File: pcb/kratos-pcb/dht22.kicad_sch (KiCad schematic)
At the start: 3 parts, among them U2 DHT22

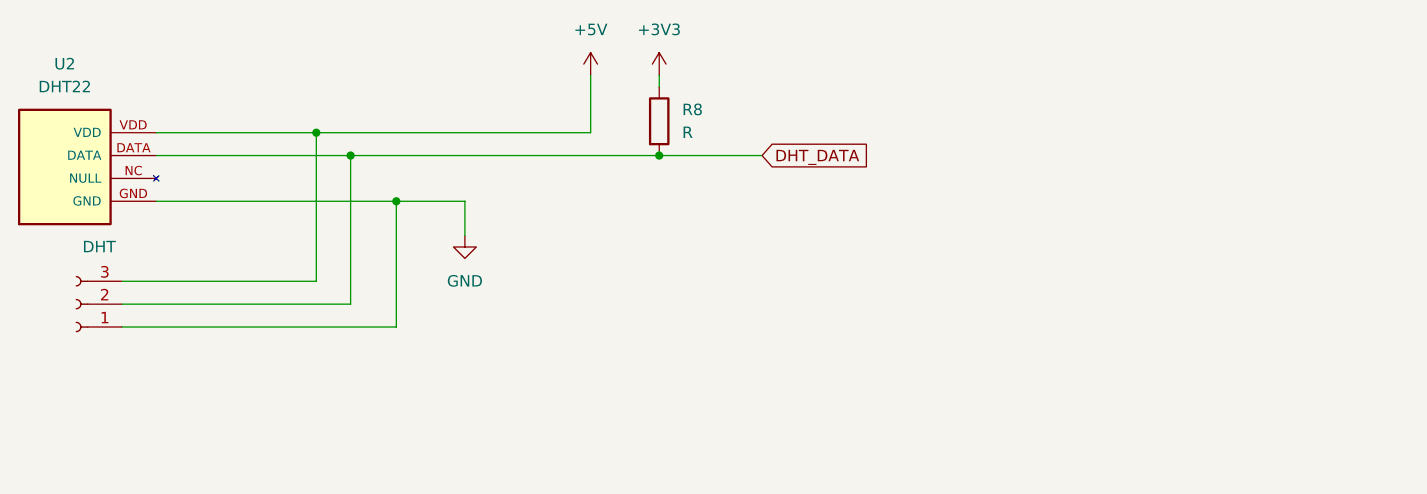
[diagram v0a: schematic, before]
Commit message: ### added
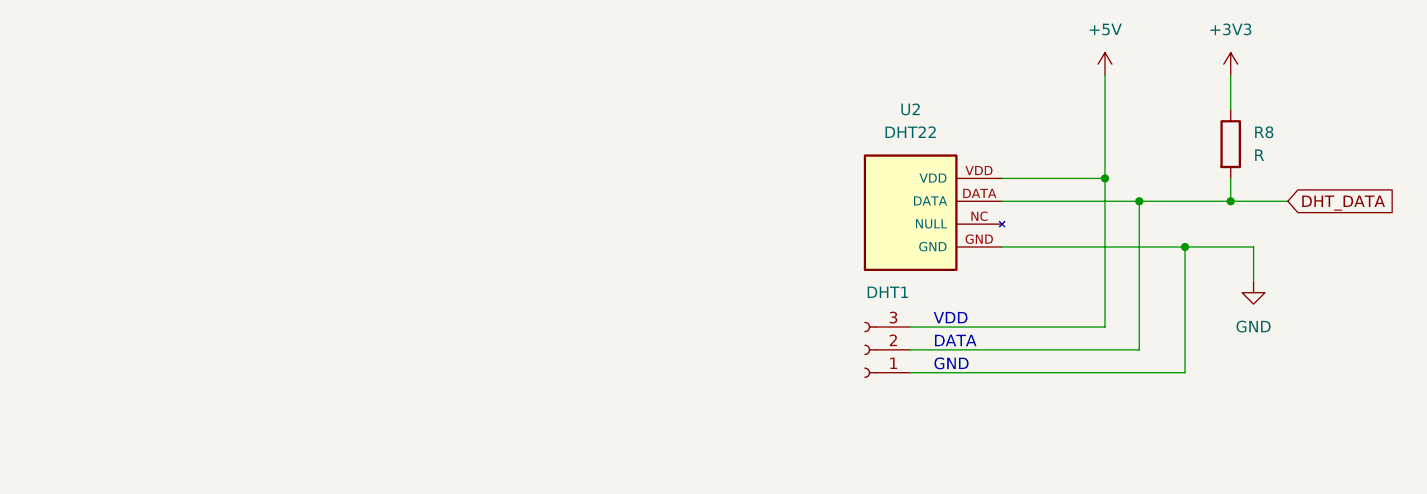
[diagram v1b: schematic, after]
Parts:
- DHT1: renamed from DHT; footprint (none) -> Connector:JWT_A3963_1x02_P3.96mm_Vertical
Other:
- note added: "DATA"
- note added: "GND"
- note added: "VDD"
- moved on the sheet: DHT1, R8, U2

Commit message: ### update     - kicad schematic
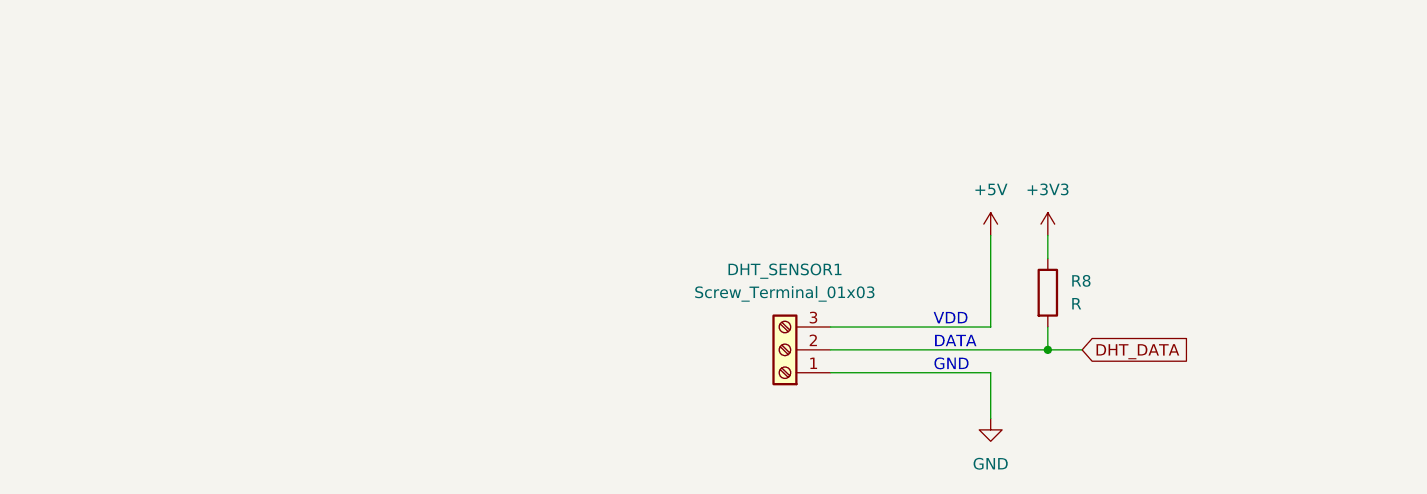
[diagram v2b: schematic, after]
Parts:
- removed DHT1: Conn_01x03_Socket, Connector:JWT_A3963_1x02_P3.96mm_Vertical, symbol Connector:Conn_01x03_Socket
- removed U2: DHT22, DHT22:DHT22, symbol DHT22:DHT22
- added DHT_SENSOR1: Screw_Terminal_01x03, TerminalBlock_4Ucon:TerminalBlock_4Ucon_1x03_P3.50mm_Horizontal, symbol Connector:Screw_Terminal_01x03
- R8: footprint (none) -> Resistor_THT:R_Axial_DIN0204_L3.6mm_D1.6mm_P5.08mm_Horizontal
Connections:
- net +5V: now also DHT_SENSOR1.3 (Pin_3)
- net DHT_DATA: now also DHT_SENSOR1.2 (Pin_2)
- net GND: now also DHT_SENSOR1.1 (Pin_1)
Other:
- moved on the sheet: R8
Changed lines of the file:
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@@
 (kicad_sch (version 20230121) (generator eeschema)
   (paper "A4")
-  (junction (at 151.13 95.25) (diameter 0) (color 0 0 0 0)
+  (junction (at 135.89 106.68) (diameter 0) (color 0 0 0 0)
   )
-  (junction (at 156.21 90.17) (diameter 0) (color 0 0 0 0)
-  )
-  (junction (at 142.24 87.63) (diameter 0) (color 0 0 0 0)
-  )
-  (junction (at 146.05 90.17) (diameter 0) (color 0 0 0 0)
-  )
-  (wire (pts (xy 146.05 106.68) (xy 146.05 90.17))
+  (wire (pts (xy 135.89 106.68) (xy 139.7 106.68))
     (stroke (width 0) (type default))
   )
-  (wire (pts (xy 120.65 104.14) (xy 142.24 104.14))
+  (wire (pts (xy 135.89 93.98) (xy 135.89 96.52))
     (stroke (width 0) (type default))
   )
-  (wire (pts (xy 130.81 90.17) (xy 146.05 90.17))
+  (wire (pts (xy 111.76 106.68) (xy 135.89 106.68))
     (stroke (width 0) (type default))
   )
-  (wire (pts (xy 151.13 95.25) (xy 130.81 95.25))
+  (wire (pts (xy 111.76 104.14) (xy 129.54 104.14))
     (stroke (width 0) (type default))
   )
-  (wire (pts (xy 130.81 87.63) (xy 142.24 87.63))
+  (wire (pts (xy 111.76 109.22) (xy 129.54 109.22))
     (stroke (width 0) (type default))
   )
-  (wire (pts (xy 146.05 90.17) (xy 156.21 90.17))
+  (wire (pts (xy 129.54 93.98) (xy 129.54 104.14))
     (stroke (width 0) (type default))
   )
-  (wire (pts (xy 120.65 109.22) (xy 151.13 109.22))
+  (wire (pts (xy 135.89 104.14) (xy 135.89 106.68))
     (stroke (width 0) (type default))
   )
-  (wire (pts (xy 142.24 87.63) (xy 142.24 76.2))
-    (stroke (width 0) (type default))
-  )
-  (wire (pts (xy 120.65 106.68) (xy 146.05 106.68))
-    (stroke (width 0) (type default))
-  )
-  (wire (pts (xy 142.24 104.14) (xy 142.24 87.63))
-    (stroke (width 0) (type default))
-  )
-  (wire (pts (xy 151.13 109.22) (xy 151.13 95.25))
-    (stroke (width 0) (type default))
-  )
-  (wire (pts (xy 158.75 95.25) (xy 151.13 95.25))
-    (stroke (width 0) (type default))
-  )
-  (wire (pts (xy 156.21 87.63) (xy 156.21 90.17))
-    (stroke (width 0) (type default))
-  )
-  (wire (pts (xy 156.21 90.17) (xy 162.56 90.17))
-    (stroke (width 0) (type default))
-  )
-  (wire (pts (xy 158.75 95.25) (xy 158.75 99.06))
-    (stroke (width 0) (type default))
-  )
-  (wire (pts (xy 156.21 76.2) (xy 156.21 80.01))
+  (wire (pts (xy 129.54 109.22) (xy 129.54 114.3))
     (stroke (width 0) (type default))
   )
@@
     (effects (font (size 1.27 1.27)) (justify left bottom))
   )
-  (global_label "DHT_DATA" (shape input) (at 162.56 90.17 0) (fields_autoplaced)
+  (global_label "DHT_DATA" (shape input) (at 139.7 106.68 0) (fields_autoplaced)
     (effects (font (size 1.27 1.27)) (justify left))
-    (property "Intersheetrefs" "${INTERSHEET_REFS}" (at 174.4957 90.17 0)
+    (property "Intersheetrefs" "${INTERSHEET_REFS}" (at 151.6357 106.68 0)
       (effects (font (size 1.27 1.27)) (justify left) hide)
     )
   )
-  (symbol (lib_id "power:GND") (at 158.75 99.06 0) (unit 1)
+  (symbol (lib_id "power:GND") (at 129.54 114.3 0) (unit 1)
     (in_bom yes) (on_board yes) (dnp no) (fields_autoplaced)
-    (property "Reference" "#PWR014" (at 158.75 105.41 0)
+    (property "Reference" "#PWR014" (at 129.54 120.65 0)
       (effects (font (size 1.27 1.27)) hide)
     )
-    (property "Value" "GND" (at 158.75 104.14 0)
+    (property "Value" "GND" (at 129.54 119.38 0)
       (effects (font (size 1.27 1.27)))
     )
-    (property "Footprint" "" (at 158.75 99.06 0)
+    (property "Footprint" "" (at 129.54 114.3 0)
       (effects (font (size 1.27 1.27)) hide)
     )
-    (property "Datasheet" "" (at 158.75 99.06 0)
+    (property "Datasheet" "" (at 129.54 114.3 0)
       (effects (font (size 1.27 1.27)) hide)
     )
@@
     )
   )
-  (symbol (lib_id "DHT22:DHT22") (at 115.57 97.79 0) (unit 1)
+  (symbol (lib_id "Connector:Screw_Terminal_01x03") (at 106.68 106.68 180) (unit 1)
     (in_bom yes) (on_board yes) (dnp no) (fields_autoplaced)
-    (property "Reference" "U2" (at 120.65 80.01 0)
+    (property "Reference" "DHT_SENSOR1" (at 106.68 97.79 0)
       (effects (font (size 1.27 1.27)))
     )
-    (property "Value" "DHT22" (at 120.65 82.55 0)
+    (property "Value" "Screw_Terminal_01x03" (at 106.68 100.33 0)
       (effects (font (size 1.27 1.27)))
     )
-    (property "Footprint" "DHT22:DHT22" (at 115.57 97.79 0)
-      (effects (font (size 1.27 1.27)) (justify bottom) hide)
-    )
-    (property "Datasheet" "" (at 115.57 97.79 0)
+    (property "Footprint" "TerminalBlock_4Ucon:TerminalBlock_4Ucon_1x03_P3.50mm_Horizontal" (at 106.68 106.68 0)
       (effects (font (size 1.27 1.27)) hide)
     )
-    (property "MF" "Aosong Electronics" (at 115.57 97.79 0)
-      (effects (font (size 1.27 1.27)) (justify bottom) hide)
+    (property "Datasheet" "~" (at 106.68 106.68 0)
+      (effects (font (size 1.27 1.27)) hide)
     )
-    (property "Description" "\nCapacitive-type humidity and temperature module/sensor\n" (at 115.57 97.79 0)
-      (effects (font (size 1.27 1.27)) (justify bottom) hide)
-    )
-    (property "Package" "Package" (at 115.57 97.79 0)
-      (effects (font (size 1.27 1.27)) (justify bottom) hide)
-    )
-    (property "Price" "None" (at 115.57 97.79 0)
-      (effects (font (size 1.27 1.27)) (justify bottom) hide)
-    )
-    (property "SnapEDA_Link" "https://www.snapeda.com/parts/DHT22/Aosong+Electronics/view-part/?ref=snap" (at 115.57 97.79 0)
-      (effects (font (size 1.27 1.27)) (justify bottom) hide)
-    )
-    (property "MP" "DHT22" (at 115.57 97.79 0)
-      (effects (font (size 1.27 1.27)) (justify bottom) hide)
-    )
-    (property "Availability" "Not in stock" (at 115.57 97.79 0)
-      (effects (font (size 1.27 1.27)) (justify bottom) hide)
-    )
-    (property "Check_prices" "https://www.snapeda.com/parts/DHT22/Aosong+Electronics/view-part/?ref=eda" (at 115.57 97.79 0)
-      (effects (font (size 1.27 1.27)) (justify bottom) hide)
-    )
-    (pin "DATA")
-    (pin "GND")
-    (pin "NC")
-    (pin "VDD")
+    (pin "2")
+    (pin "1")
+    (pin "3")
     (instances
       (project "kratos-pcb"
         (path "/12f1b997-8c5f-4ef7-b036-7873ddaba48e/ab0aa194-5f27-4f16-bd8b-12afa764e651"
-          (reference "U2") (unit 1)
+          (reference "DHT_SENSOR1") (unit 1)
         )
       )
     )
   )
-  (symbol (lib_id "Connector:Conn_01x03_Socket") (at 115.57 106.68 180) (unit 1)
-    (in_bom yes) (on_board yes) (dnp no)
-    (property "Reference" "DHT1" (at 118.11 100.33 0)
+  (symbol (lib_id "power:+3V3") (at 135.89 93.98 0) (unit 1)
+    (in_bom yes) (on_board yes) (dnp no) (fields_autoplaced)
+    (property "Reference" "#PWR012" (at 135.89 97.79 0)
+      (effects (font (size 1.27 1.27)) hide)
+    )
+    (property "Value" "+3V3" (at 135.89 88.9 0)
       (effects (font (size 1.27 1.27)))
     )
-    (property "Value" "Conn_01x03_Socket" (at 110.49 101.6 0)
+    (property "Footprint" "" (at 135.89 93.98 0)
       (effects (font (size 1.27 1.27)) hide)
     )
-    (property "Footprint" "Connector:JWT_A3963_1x02_P3.96mm_Vertical" (at 115.57 106.68 0)
-      (effects (font (size 1.27 1.27)) hide)
-    )
-    (property "Datasheet" "~" (at 115.57 106.68 0)
-      (effects (font (size 1.27 1.27)) hide)
-    )
-    (pin "3")
-    (pin "2")
-    (pin "1")
-    (instances
-      (project "kratos-pcb"
-        (path "/12f1b997-8c5f-4ef7-b036-7873ddaba48e/ab0aa194-5f27-4f16-bd8b-12afa764e651"
-          (reference "DHT1") (unit 1)
-        )
-      )
-    )
-  )
-  (symbol (lib_id "power:+3V3") (at 156.21 76.2 0) (unit 1)
-    (in_bom yes) (on_board yes) (dnp no) (fields_autoplaced)
-    (property "Reference" "#PWR012" (at 156.21 80.01 0)
-      (effects (font (size 1.27 1.27)) hide)
-    )
-    (property "Value" "+3V3" (at 156.21 71.12 0)
-      (effects (font (size 1.27 1.27)))
-    )
-    (property "Footprint" "" (at 156.21 76.2 0)
-      (effects (font (size 1.27 1.27)) hide)
-    )
-    (property "Datasheet" "" (at 156.21 76.2 0)
+    (property "Datasheet" "" (at 135.89 93.98 0)
       (effects (font (size 1.27 1.27)) hide)
     )
@@
     )
   )
-  (symbol (lib_id "Device:R") (at 156.21 83.82 0) (unit 1)
+  (symbol (lib_id "Device:R") (at 135.89 100.33 0) (unit 1)
     (in_bom yes) (on_board yes) (dnp no) (fields_autoplaced)
-    (property "Reference" "R8" (at 158.75 82.55 0)
+    (property "Reference" "R8" (at 138.43 99.06 0)
       (effects (font (size 1.27 1.27)) (justify left))
     )
-    (property "Value" "R" (at 158.75 85.09 0)
+    (property "Value" "R" (at 138.43 101.6 0)
       (effects (font (size 1.27 1.27)) (justify left))
     )
-    (property "Footprint" "" (at 154.432 83.82 90)
+    (property "Footprint" "Resistor_THT:R_Axial_DIN0204_L3.6mm_D1.6mm_P5.08mm_Horizontal" (at 134.112 100.33 90)
       (effects (font (size 1.27 1.27)) hide)
     )
-    (property "Datasheet" "~" (at 156.21 83.82 0)
+    (property "Datasheet" "~" (at 135.89 100.33 0)
       (effects (font (size 1.27 1.27)) hide)
     )
@@
     )
   )
-  (symbol (lib_id "power:+5V") (at 142.24 76.2 0) (unit 1)
+  (symbol (lib_id "power:+5V") (at 129.54 93.98 0) (unit 1)
     (in_bom yes) (on_board yes) (dnp no) (fields_autoplaced)
-    (property "Reference" "#PWR013" (at 142.24 80.01 0)
+    (property "Reference" "#PWR013" (at 129.54 97.79 0)
       (effects (font (size 1.27 1.27)) hide)
     )
-    (property "Value" "+5V" (at 142.24 71.12 0)
+    (property "Value" "+5V" (at 129.54 88.9 0)
       (effects (font (size 1.27 1.27)))
     )
-    (property "Footprint" "" (at 142.24 76.2 0)
+    (property "Footprint" "" (at 129.54 93.98 0)
       (effects (font (size 1.27 1.27)) hide)
     )
-    (property "Datasheet" "" (at 142.24 76.2 0)
+    (property "Datasheet" "" (at 129.54 93.98 0)
       (effects (font (size 1.27 1.27)) hide)
     )

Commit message: kicad
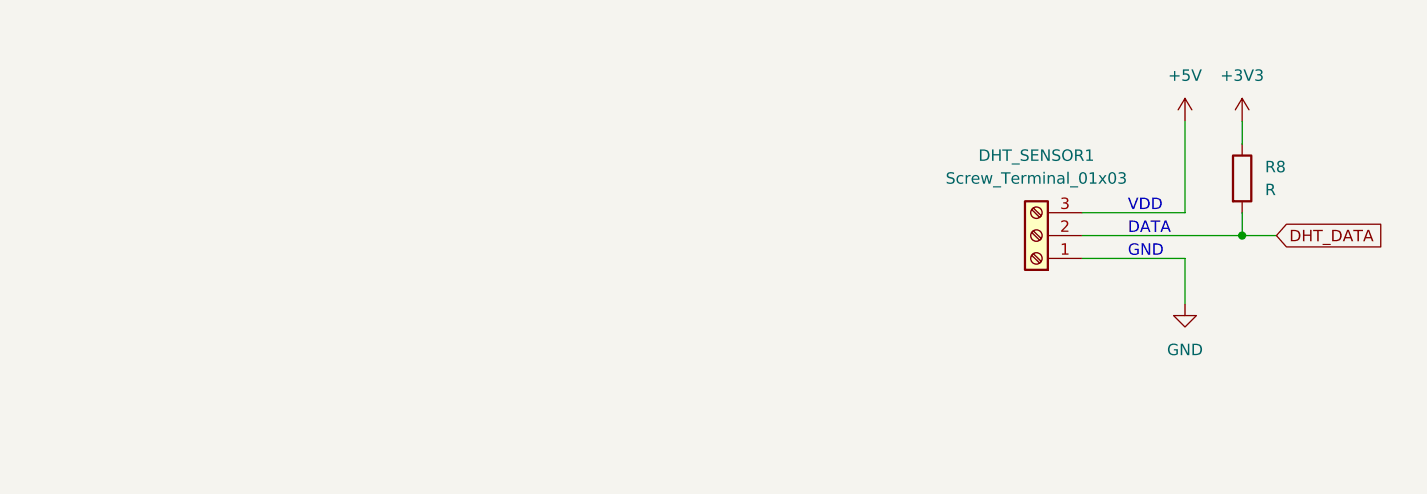
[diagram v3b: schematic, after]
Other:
- moved on the sheet: DHT_SENSOR1, R8
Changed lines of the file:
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@@
 (kicad_sch (version 20230121) (generator eeschema)
   (paper "A4")
-  (junction (at 135.89 106.68) (diameter 0) (color 0 0 0 0)
+  (junction (at 157.48 93.98) (diameter 0) (color 0 0 0 0)
   )
-  (wire (pts (xy 135.89 106.68) (xy 139.7 106.68))
+  (wire (pts (xy 157.48 81.28) (xy 157.48 83.82))
     (stroke (width 0) (type default))
   )
-  (wire (pts (xy 135.89 93.98) (xy 135.89 96.52))
+  (wire (pts (xy 139.7 93.98) (xy 157.48 93.98))
     (stroke (width 0) (type default))
   )
-  (wire (pts (xy 111.76 106.68) (xy 135.89 106.68))
+  (wire (pts (xy 139.7 91.44) (xy 151.13 91.44))
     (stroke (width 0) (type default))
   )
-  (wire (pts (xy 111.76 104.14) (xy 129.54 104.14))
+  (wire (pts (xy 157.48 93.98) (xy 161.29 93.98))
     (stroke (width 0) (type default))
   )
-  (wire (pts (xy 111.76 109.22) (xy 129.54 109.22))
+  (wire (pts (xy 139.7 96.52) (xy 151.13 96.52))
     (stroke (width 0) (type default))
   )
-  (wire (pts (xy 129.54 93.98) (xy 129.54 104.14))
+  (wire (pts (xy 151.13 81.28) (xy 151.13 91.44))
     (stroke (width 0) (type default))
   )
-  (wire (pts (xy 135.89 104.14) (xy 135.89 106.68))
+  (wire (pts (xy 157.48 91.44) (xy 157.48 93.98))
     (stroke (width 0) (type default))
   )
-  (wire (pts (xy 129.54 109.22) (xy 129.54 114.3))
+  (wire (pts (xy 151.13 96.52) (xy 151.13 101.6))
     (stroke (width 0) (type default))
   )
-  (text "VDD" (at 123.19 104.14 0)
+  (text "VDD" (at 144.78 91.44 0)
     (effects (font (size 1.27 1.27)) (justify left bottom))
   )
-  (text "DATA" (at 123.19 106.68 0)
+  (text "DATA" (at 144.78 93.98 0)
     (effects (font (size 1.27 1.27)) (justify left bottom))
   )
-  (text "GND" (at 123.19 109.22 0)
+  (text "GND" (at 144.78 96.52 0)
     (effects (font (size 1.27 1.27)) (justify left bottom))
   )
-  (global_label "DHT_DATA" (shape input) (at 139.7 106.68 0) (fields_autoplaced)
+  (global_label "DHT_DATA" (shape input) (at 161.29 93.98 0) (fields_autoplaced)
     (effects (font (size 1.27 1.27)) (justify left))
-    (property "Intersheetrefs" "${INTERSHEET_REFS}" (at 151.6357 106.68 0)
+    (property "Intersheetrefs" "${INTERSHEET_REFS}" (at 173.2257 93.98 0)
       (effects (font (size 1.27 1.27)) (justify left) hide)
     )
   )
-  (symbol (lib_id "power:GND") (at 129.54 114.3 0) (unit 1)
+  (symbol (lib_id "power:GND") (at 151.13 101.6 0) (unit 1)
     (in_bom yes) (on_board yes) (dnp no) (fields_autoplaced)
-    (property "Reference" "#PWR014" (at 129.54 120.65 0)
+    (property "Reference" "#PWR014" (at 151.13 107.95 0)
       (effects (font (size 1.27 1.27)) hide)
     )
-    (property "Value" "GND" (at 129.54 119.38 0)
+    (property "Value" "GND" (at 151.13 106.68 0)
       (effects (font (size 1.27 1.27)))
     )
-    (property "Footprint" "" (at 129.54 114.3 0)
+    (property "Footprint" "" (at 151.13 101.6 0)
       (effects (font (size 1.27 1.27)) hide)
     )
-    (property "Datasheet" "" (at 129.54 114.3 0)
+    (property "Datasheet" "" (at 151.13 101.6 0)
       (effects (font (size 1.27 1.27)) hide)
     )
@@
     )
   )
-  (symbol (lib_id "Connector:Screw_Terminal_01x03") (at 106.68 106.68 180) (unit 1)
+  (symbol (lib_id "Connector:Screw_Terminal_01x03") (at 134.62 93.98 180) (unit 1)
     (in_bom yes) (on_board yes) (dnp no) (fields_autoplaced)
-    (property "Reference" "DHT_SENSOR1" (at 106.68 97.79 0)
+    (property "Reference" "DHT_SENSOR1" (at 134.62 85.09 0)
       (effects (font (size 1.27 1.27)))
     )
-    (property "Value" "Screw_Terminal_01x03" (at 106.68 100.33 0)
+    (property "Value" "Screw_Terminal_01x03" (at 134.62 87.63 0)
       (effects (font (size 1.27 1.27)))
     )
-    (property "Footprint" "TerminalBlock_4Ucon:TerminalBlock_4Ucon_1x03_P3.50mm_Horizontal" (at 106.68 106.68 0)
+    (property "Footprint" "TerminalBlock_4Ucon:TerminalBlock_4Ucon_1x03_P3.50mm_Horizontal" (at 134.62 93.98 0)
       (effects (font (size 1.27 1.27)) hide)
     )
-    (property "Datasheet" "~" (at 106.68 106.68 0)
+    (property "Datasheet" "~" (at 134.62 93.98 0)
       (effects (font (size 1.27 1.27)) hide)
     )
@@
     )
   )
-  (symbol (lib_id "power:+3V3") (at 135.89 93.98 0) (unit 1)
+  (symbol (lib_id "power:+3V3") (at 157.48 81.28 0) (unit 1)
     (in_bom yes) (on_board yes) (dnp no) (fields_autoplaced)
-    (property "Reference" "#PWR012" (at 135.89 97.79 0)
+    (property "Reference" "#PWR012" (at 157.48 85.09 0)
       (effects (font (size 1.27 1.27)) hide)
     )
-    (property "Value" "+3V3" (at 135.89 88.9 0)
+    (property "Value" "+3V3" (at 157.48 76.2 0)
       (effects (font (size 1.27 1.27)))
     )
-    (property "Footprint" "" (at 135.89 93.98 0)
+    (property "Footprint" "" (at 157.48 81.28 0)
       (effects (font (size 1.27 1.27)) hide)
     )
-    (property "Datasheet" "" (at 135.89 93.98 0)
+    (property "Datasheet" "" (at 157.48 81.28 0)
       (effects (font (size 1.27 1.27)) hide)
     )
@@
     )
   )
-  (symbol (lib_id "Device:R") (at 135.89 100.33 0) (unit 1)
+  (symbol (lib_id "Device:R") (at 157.48 87.63 0) (unit 1)
     (in_bom yes) (on_board yes) (dnp no) (fields_autoplaced)
-    (property "Reference" "R8" (at 138.43 99.06 0)
+    (property "Reference" "R8" (at 160.02 86.36 0)
       (effects (font (size 1.27 1.27)) (justify left))
     )
-    (property "Value" "R" (at 138.43 101.6 0)
+    (property "Value" "R" (at 160.02 88.9 0)
       (effects (font (size 1.27 1.27)) (justify left))
     )
-    (property "Footprint" "Resistor_THT:R_Axial_DIN0204_L3.6mm_D1.6mm_P5.08mm_Horizontal" (at 134.112 100.33 90)
+    (property "Footprint" "Resistor_THT:R_Axial_DIN0204_L3.6mm_D1.6mm_P5.08mm_Horizontal" (at 155.702 87.63 90)
       (effects (font (size 1.27 1.27)) hide)
     )
-    (property "Datasheet" "~" (at 135.89 100.33 0)
+    (property "Datasheet" "~" (at 157.48 87.63 0)
       (effects (font (size 1.27 1.27)) hide)
     )
@@
     )
   )
-  (symbol (lib_id "power:+5V") (at 129.54 93.98 0) (unit 1)
+  (symbol (lib_id "power:+5V") (at 151.13 81.28 0) (unit 1)
     (in_bom yes) (on_board yes) (dnp no) (fields_autoplaced)
-    (property "Reference" "#PWR013" (at 129.54 97.79 0)
+    (property "Reference" "#PWR013" (at 151.13 85.09 0)
       (effects (font (size 1.27 1.27)) hide)
     )
-    (property "Value" "+5V" (at 129.54 88.9 0)
+    (property "Value" "+5V" (at 151.13 76.2 0)
       (effects (font (size 1.27 1.27)))
     )
-    (property "Footprint" "" (at 129.54 93.98 0)
+    (property "Footprint" "" (at 151.13 81.28 0)
       (effects (font (size 1.27 1.27)) hide)
     )
-    (property "Datasheet" "" (at 129.54 93.98 0)
+    (property "Datasheet" "" (at 151.13 81.28 0)
       (effects (font (size 1.27 1.27)) hide)
     )
